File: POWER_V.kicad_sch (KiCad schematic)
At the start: 29 parts, among them CN1 XT30PW-M, CN2 XT30PW-M, Q2 AOD4185_C400894, Q3 AOD4185_C400894, SW3 SWITCH_BLACK, SW4 SWITCH_BLACK, U7 TPS62901RPJR

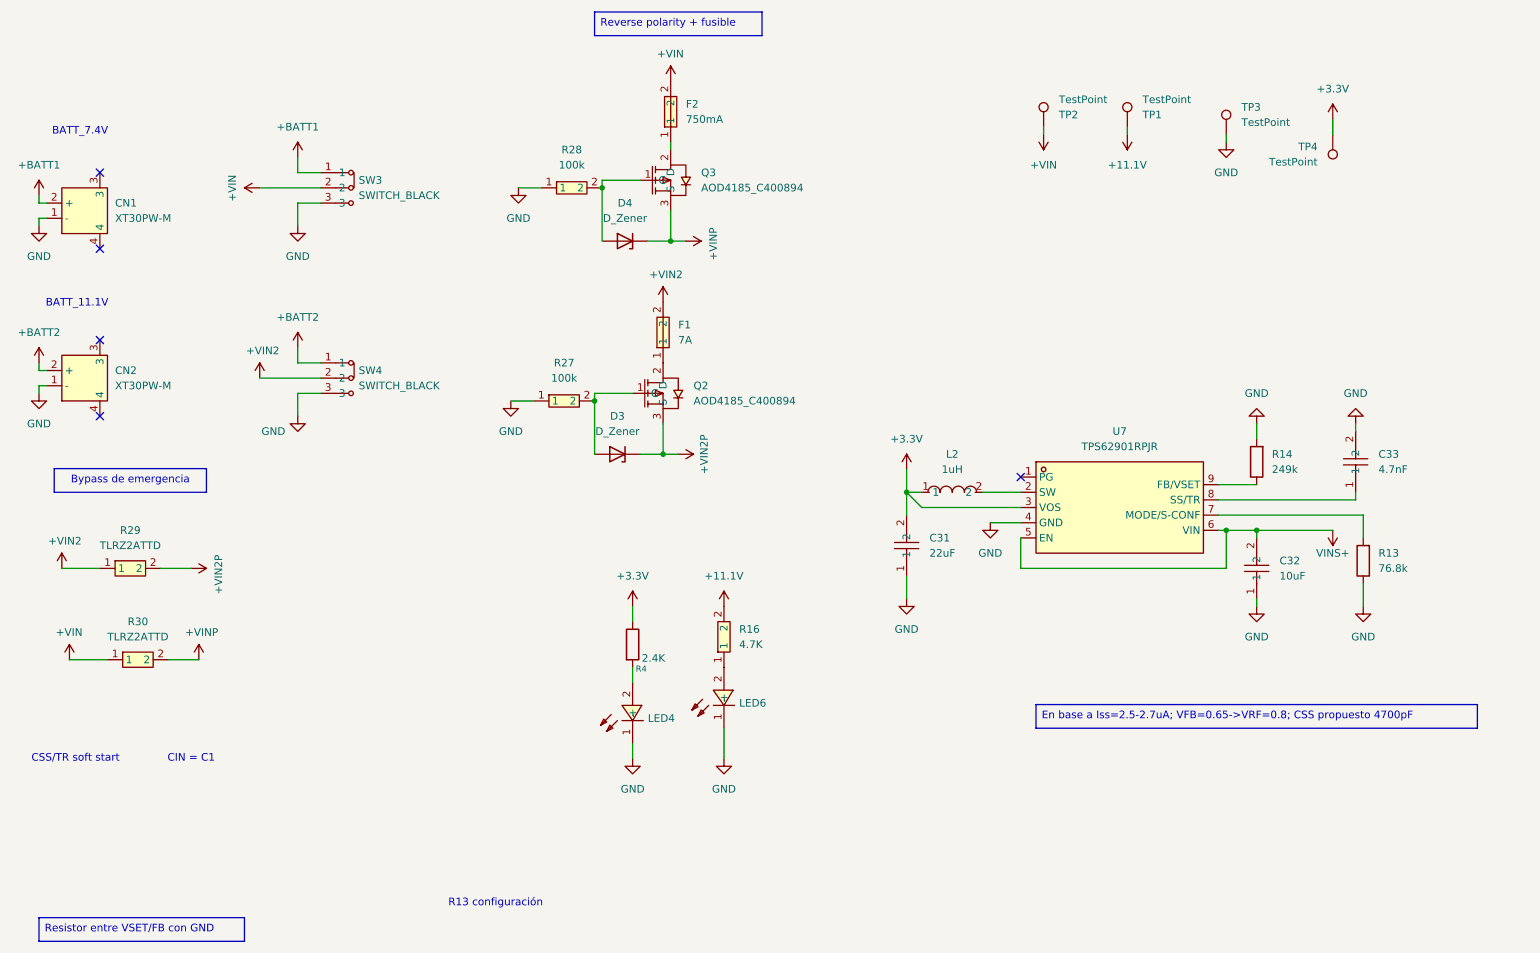
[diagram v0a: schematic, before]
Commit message: PCB_V1
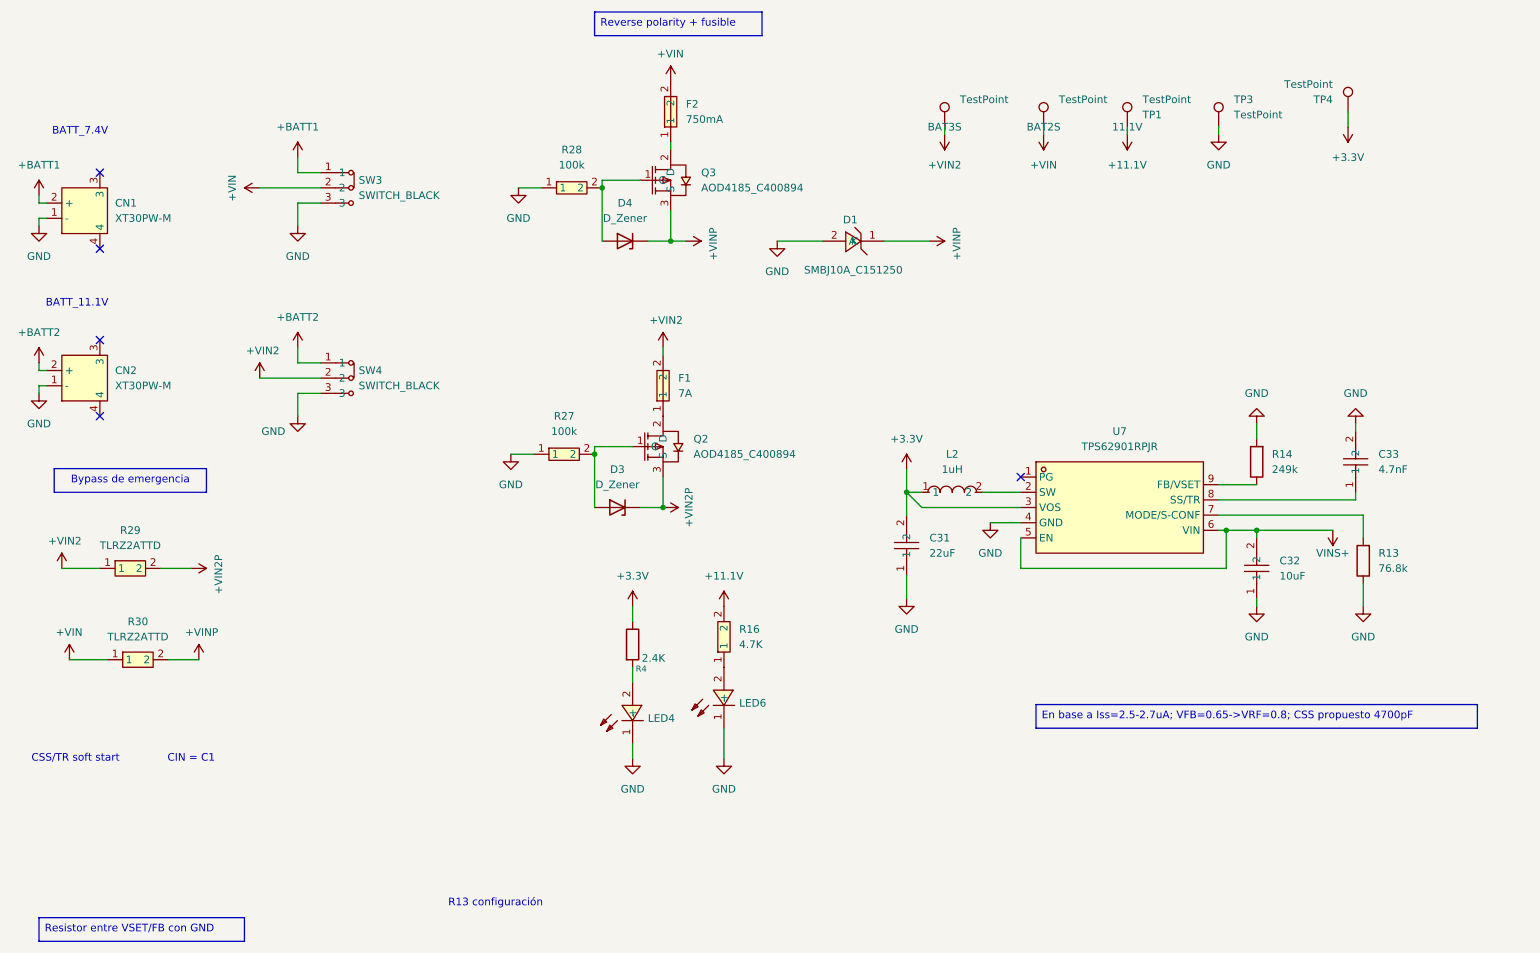
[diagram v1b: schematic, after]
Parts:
- added D1: SMBJ10A_C151250, ARLISS-footprints:SMB_L4.6-W3.6-LS5.3-RD, symbol CANSAT_STM32_symbols:SMBJ10A_C151250
- added TP5: TestPoint, TestPoint:TestPoint_Pad_D1.5mm, symbol Connector:TestPoint
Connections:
- net +VIN2: now also TP5.1
- net +VINP: now also D1.1 (K)
- net GND: now also D1.2 (A)
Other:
- moved on the sheet: D3, F1, Q2, R27, TP3, TP4
